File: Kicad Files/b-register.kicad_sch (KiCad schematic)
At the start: 20 parts, among them U29 74LS245, U30 74LS173, U31 74LS173

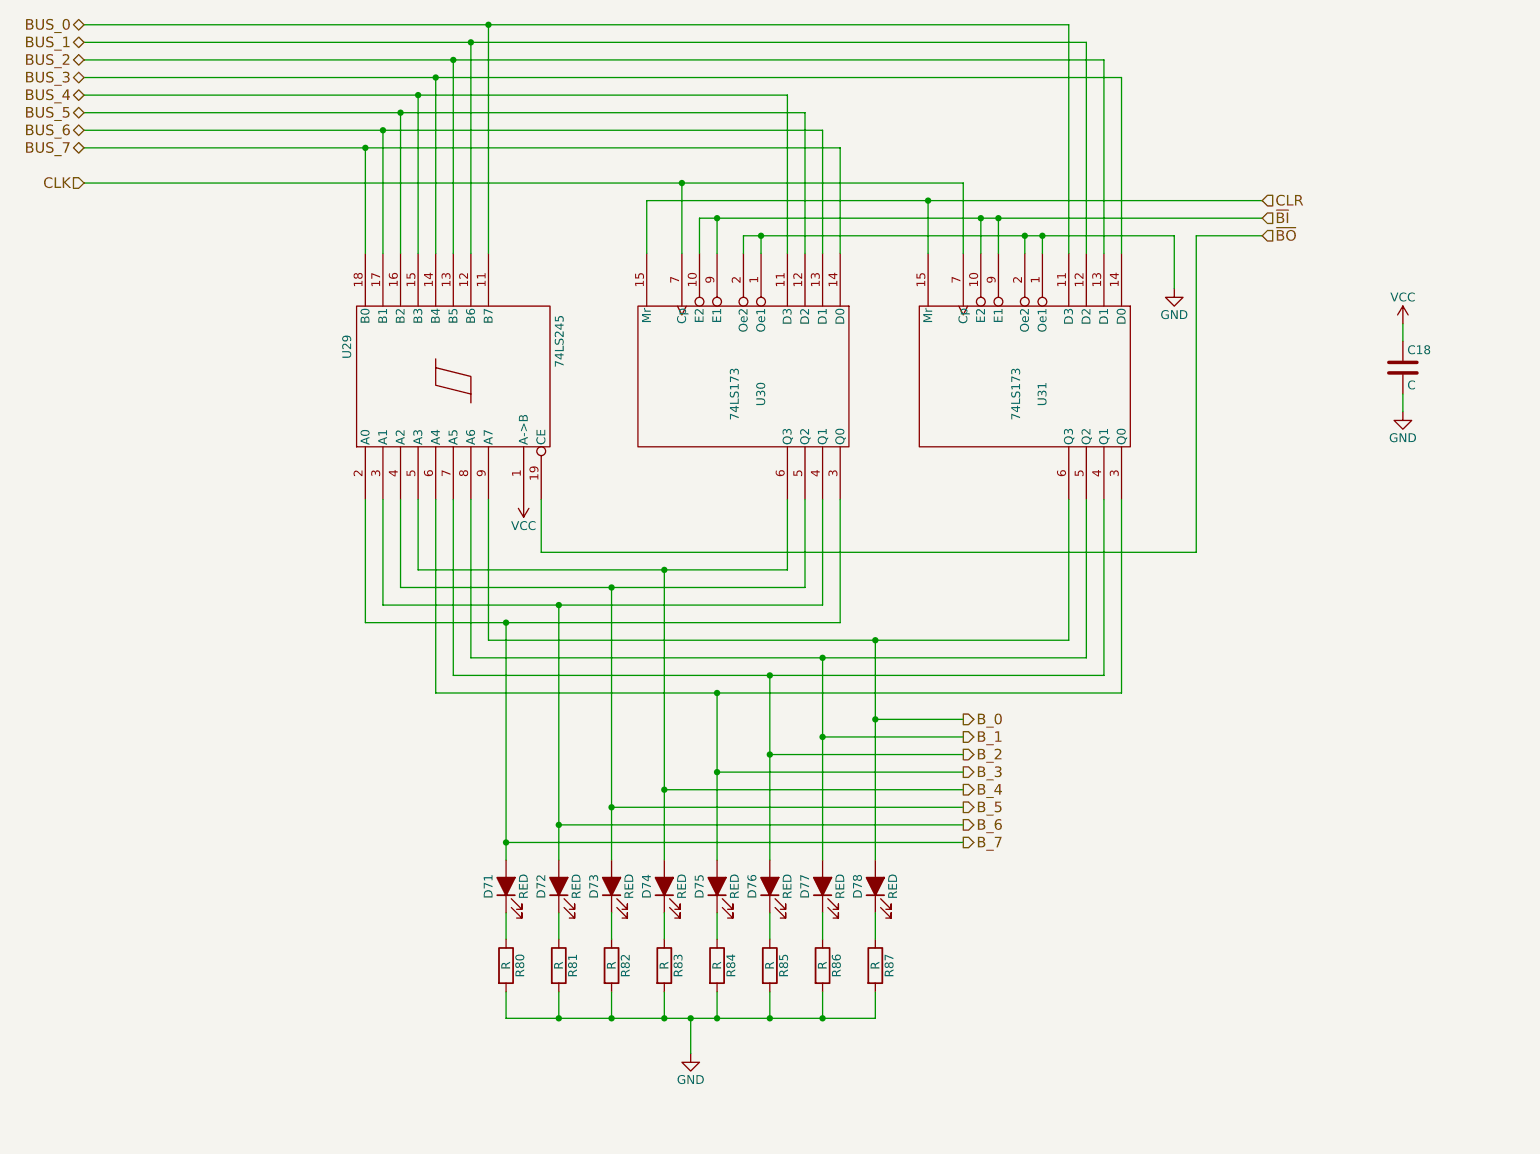
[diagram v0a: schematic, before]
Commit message: updated library
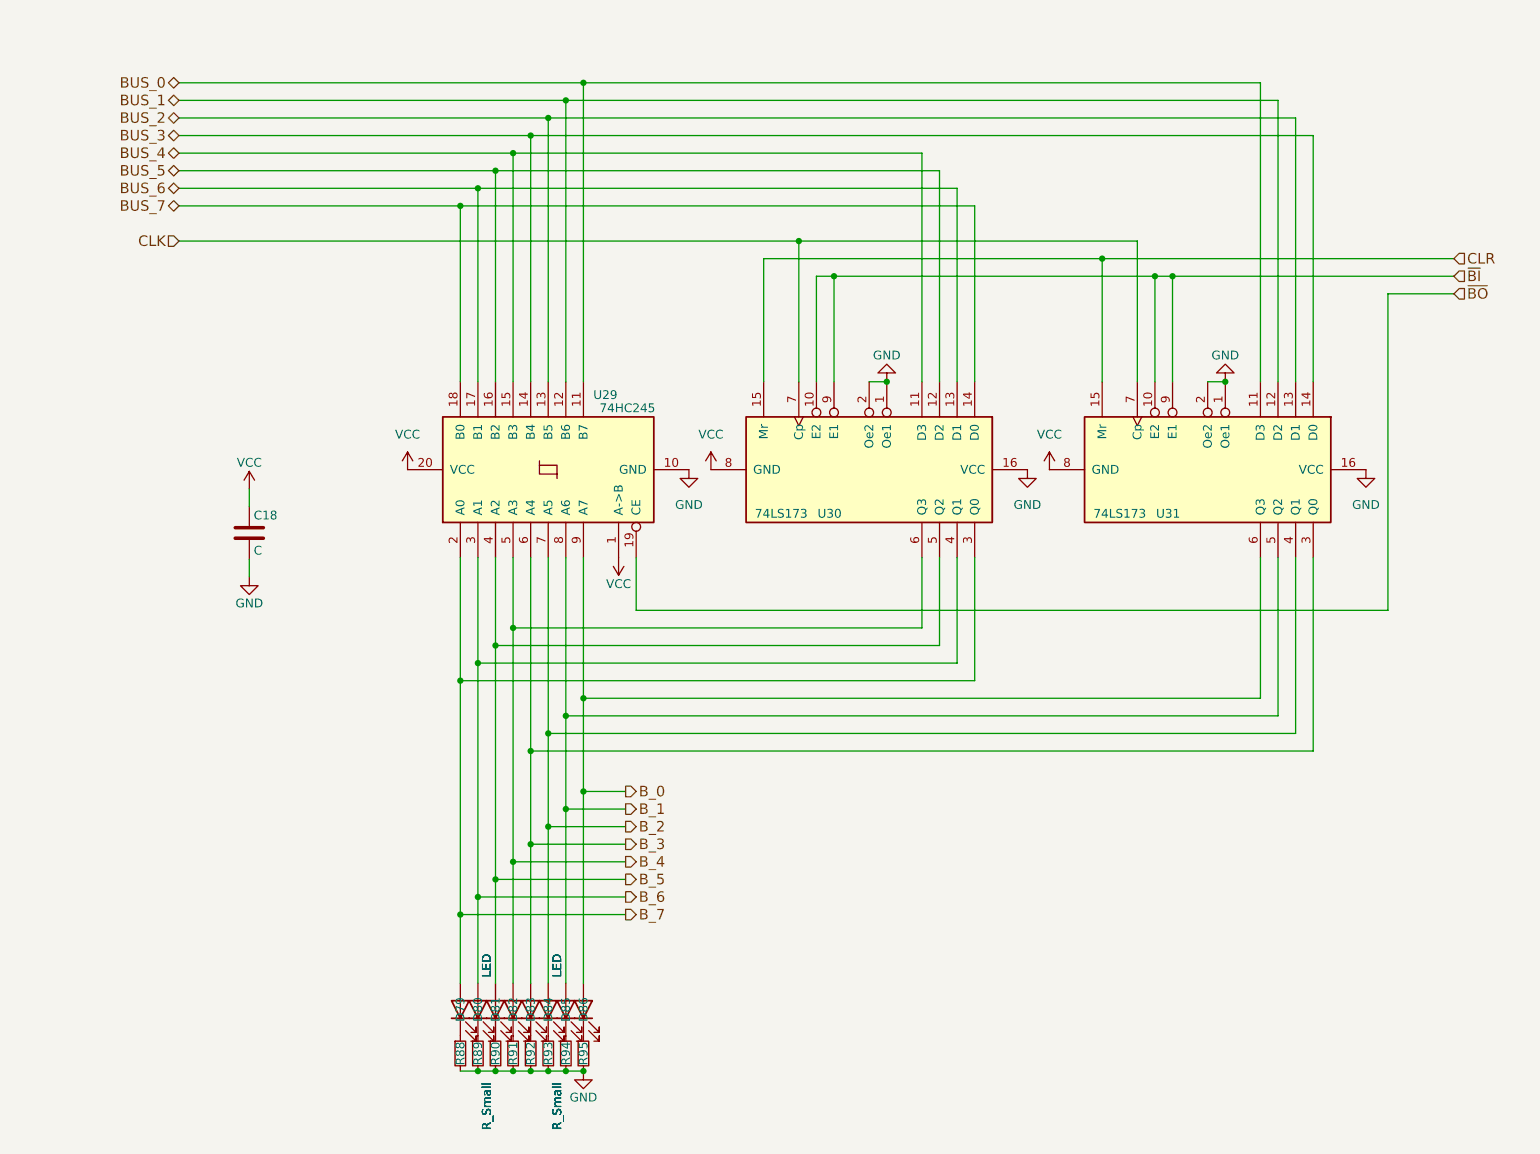
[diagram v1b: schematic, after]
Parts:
- removed D71, D72, D73, D74, D75, D76, D77, D78: RED, LED_THT:LED_D5.0mm, symbol 8bit-computer-rescue:LED_ALT-Device
- removed R80, R81, R82, R83, R84, R85, R86, R87: R, Resistor_THT:R_Axial_DIN0207_L6.3mm_D2.5mm_P7.62mm_Horizontal, symbol Device:R
- removed U29: 74LS245, Package_DIP:DIP-20_W7.62mm, symbol 8bit-computer-rescue:74LS245-8bit-computer-rescue
- removed U30, U31: 74LS173, Package_DIP:DIP-16_W7.62mm, symbol 8bit-computer-rescue:74LS173-8bit-computer-rescue
- added D79, D80, D81, D82, D83, D84, D85, D86: LED, symbol Device:LED
- added R88, R89, R90, R91, R92, R93, R94, R95: R_Small, symbol Device:R_Small
- added U29: 74HC245, symbol 74xx:74HC245
- added U30, U31: 74LS173, symbol 74xx:74LS173
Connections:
- net BUS_0: now also U29.11 (B7), U31.11 (D3)
- net BUS_1: now also U29.12 (B6), U31.12 (D2)
- net BUS_2: now also U29.13 (B5), U31.13 (D1)
- net BUS_3: now also U29.14 (B4), U31.14 (D0)
- net BUS_4: now also U29.15 (B3), U30.11 (D3)
- net BUS_5: now also U29.16 (B2), U30.12 (D2)
- net BUS_6: now also U29.17 (B1), U30.13 (D1)
- net BUS_7: now also U29.18 (B0), U30.14 (D0)
- net B_0: now also D86.2 (A), U29.9 (A7), U31.6 (Q3)
- net B_1: now also D85.2 (A), U29.8 (A6), U31.5 (Q2)
- net B_2: now also D84.2 (A), U29.7 (A5), U31.4 (Q1)
- net B_3: now also D83.2 (A), U29.6 (A4), U31.3 (Q0)
- net B_4: now also D82.2 (A), U29.5 (A3), U30.6 (Q3)
- net B_5: now also D81.2 (A), U29.4 (A2), U30.5 (Q2)
- net B_6: now also D80.2 (A), U29.3 (A1), U30.4 (Q1)
- net B_7: now also D79.2 (A), U29.2 (A0), U30.3 (Q0)
- net CLK: now also U30.7 (Cp), U31.7 (Cp)
- net CLR: now also U30.15 (Mr), U31.15 (Mr)
- net GND: now also R88.2, R89.2, R90.2, R91.2, R92.2, R93.2, R94.2, R95.2, U29.10 (GND), U30.1 (Oe1), U30.16 (VCC), U30.2 (Oe2), U31.1 (Oe1), U31.16 (VCC), U31.2 (Oe2)
- net VCC: now also U29.1 (A->B), U29.20 (VCC), U30.8 (GND), U31.8 (GND)
- net ~{BI}: now also U30.10 (E2), U30.9 (E1), U31.10 (E2), U31.9 (E1)
- net ~{BO}: now also U29.19 (CE)
- new net: D80.1 (K), R89.1
- new net: D81.1 (K), R90.1
- new net: D84.1 (K), R93.1
- new net: D82.1 (K), R91.1
- new net: D79.1 (K), R88.1
- new net: D83.1 (K), R92.1
- new net: D85.1 (K), R94.1
- new net: D86.1 (K), R95.1
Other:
- moved on the sheet: C18

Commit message: im sooo stupiiid
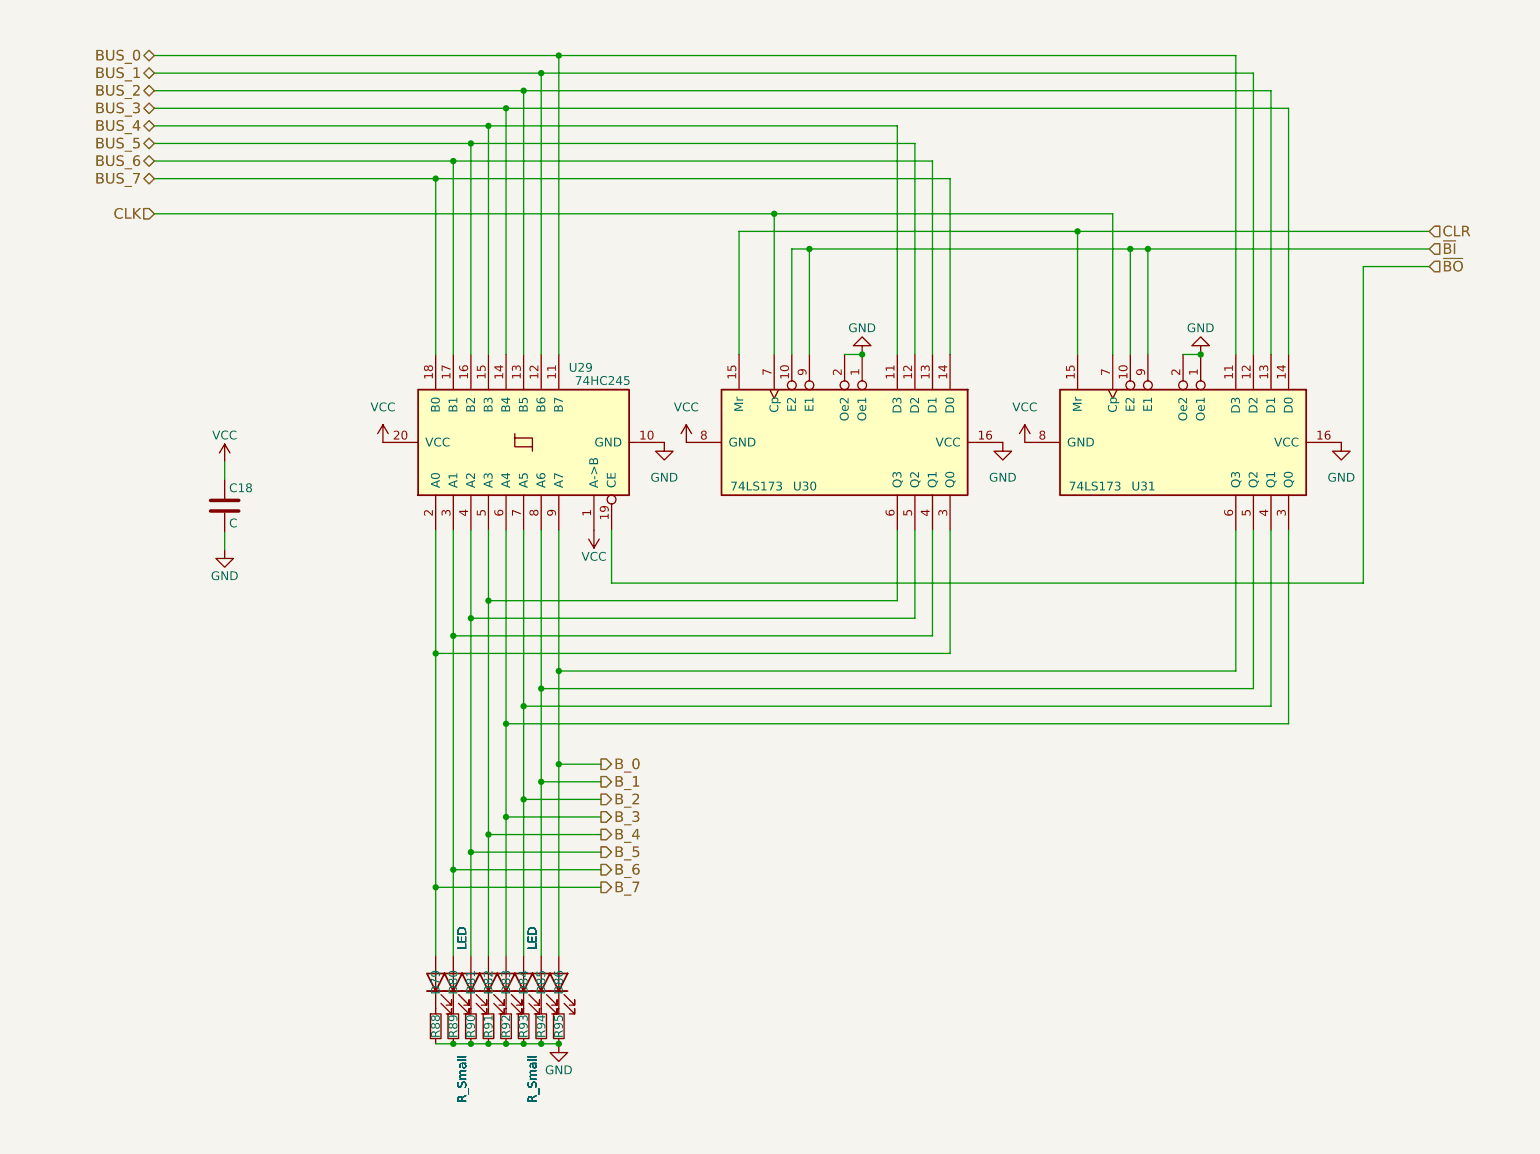
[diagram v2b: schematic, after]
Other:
- moved on the sheet: C18, D79, D80, D81, D82, D83, D84, D85, D86, R88, R89, R90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
